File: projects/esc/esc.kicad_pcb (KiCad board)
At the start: 2 copper layers, 41 parts, among them IC1 ATMEGA48-A, P1 INPUT, P2 OUTPUT, Q1 Q_NMOS_GSD, Q2 Q_NMOS_GSD, Q3 Q_NMOS_GSD, Q4 Q_NMOS_GSD, Q5 Q_NMOS_GSD, Q6 Q_NMOS_GSD, U1 74LS08, U2 74LS08

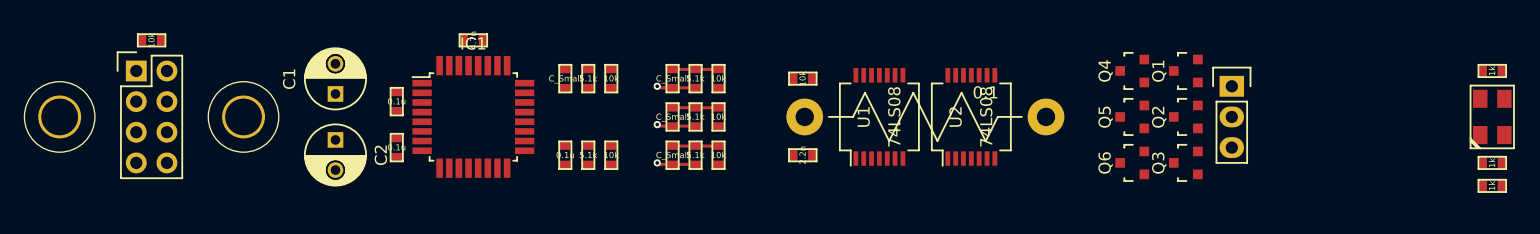
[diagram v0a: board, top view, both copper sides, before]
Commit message: fits into .5 x 3.9
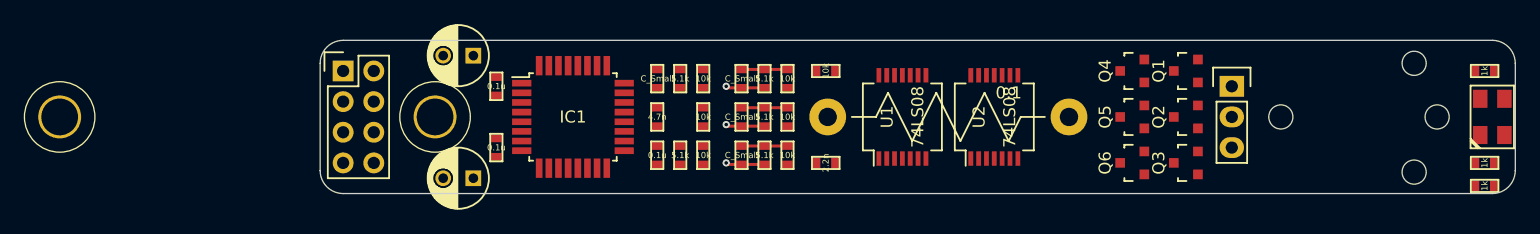
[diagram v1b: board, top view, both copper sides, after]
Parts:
- added REF**: 1pin, Connect:1pin, F.Cu at (267.2, 97.2)
- added REF**: 1pin, Connect:1pin, F.Cu at (267.2, 106.2)
- added REF**: 1pin, Connect:1pin, F.Cu at (256.2, 101.6)
- added REF**: 1pin, Connect:1pin, F.Cu at (269.1, 101.6)
- moved R12 46.2 mm to (208.3, 101.6), turned to 270 degrees
- moved P1 17.1 mm to (178.4, 97.8)
- moved C3 16.5 mm to (204.5, 101.6), turned to 90 degrees
- moved MP2 15.9 mm to (186.1, 101.6)
- moved C2 11.9 mm to (189.2, 106.7), turned to 180 degrees
- moved C1 11.9 mm to (189.2, 96.5), turned to 180 degrees
- moved C4 8.35 mm to (191.1, 99.1)
- moved IC1 8.26 mm to (197.5, 101.6)
- moved C6 8.25 mm to (191.1, 104.1)
- moved C5 7.62 mm to (204.5, 104.8)
- moved C7 7.62 mm to (204.5, 98.4)
- moved R1 7.62 mm to (208.3, 104.8)
- moved R2 7.62 mm to (206.4, 104.8)
- moved R3 7.62 mm to (208.3, 98.4)
- moved R4 7.62 mm to (206.4, 98.4)
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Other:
- board outline added: 99.1 x 12.7 mm
